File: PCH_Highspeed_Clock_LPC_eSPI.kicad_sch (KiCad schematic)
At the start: 1 part

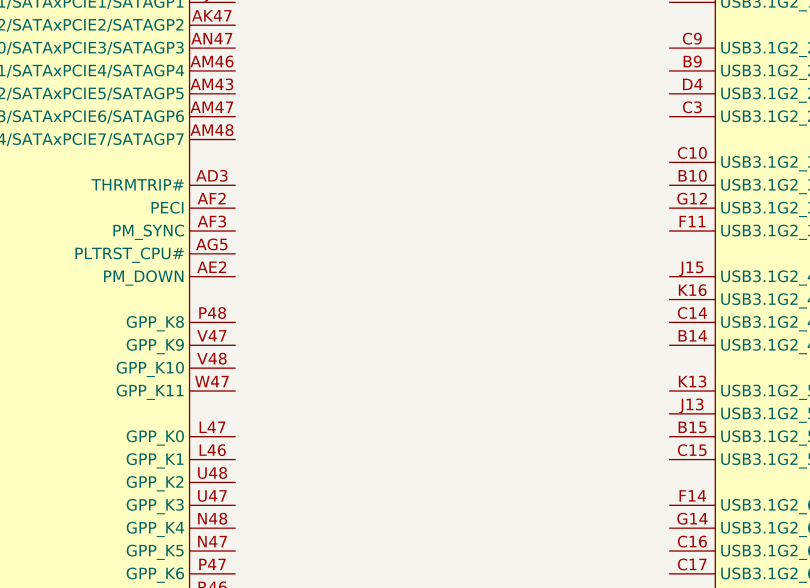
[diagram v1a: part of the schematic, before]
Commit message: implemented some misc cpu signals
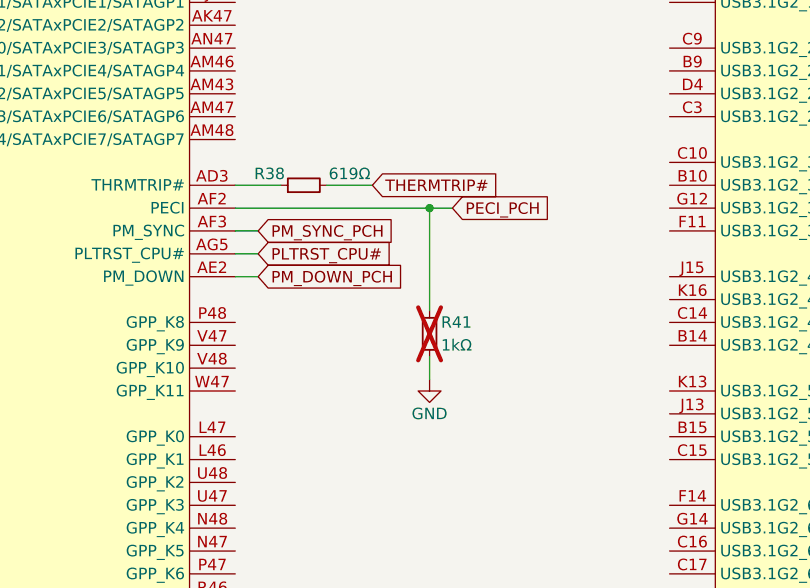
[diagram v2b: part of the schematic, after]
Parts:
- added R38: 619Ω, Resistor_SMD:R_0402_1005Metric, symbol Device:R_Small
- added R41: 1kΩ, Resistor_SMD:R_0402_1005Metric, symbol Device:R_Small
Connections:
- net at UPCH1.AD3 (THRMTRIP#): now also R38.1
- net PM_DOWN_PCH: now reaches UPCH1.AE2 (PM_DOWN)
- net PECI_PCH: now reaches UPCH1.AF2 (PECI)
- net PECI_PCH: now also R41.2
- net PM_SYNC_PCH: now reaches UPCH1.AF3 (PM_SYNC)
- net PLTRST_CPU#: now reaches UPCH1.AG5 (PLTRST_CPU#)
- new net GND: R41.1
- new net THERMTRIP#: R38.2

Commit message: idek what i changed anymore but there's a bunch of new stuff lol
iirc i did some more misc cpu pins and a bunch of pch pcie stuff
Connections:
- net SSD0_Refclk+: now reaches UPCH1.AH10 (CLKOUT_PCIE_P1)
- net SSD0_Refclk-: now reaches UPCH1.AH9 (CLKOUT_PCIE_N1)
- net SSD0_CLKREQ#: now reaches UPCH1.BE31 (GPP_B6/SRCCLKREQ1#)
- net SSD0_PCIe_Tx2+: now reaches UPCH1.B35 (PCIE10_TXP)
- net SSD0_PCIe_Tx1-: now reaches UPCH1.B36 (PCIE11_TXN/SATA0A_TXN)
- net SSD0_PCIe_Tx3-: now reaches UPCH1.C34 (PCIE9_TXN)
- net SSD0_PCIe_Tx2-: now reaches UPCH1.C35 (PCIE10_TXN)
- net SSD0_PCIe_Tx1+: now reaches UPCH1.C36 (PCIE11_TXP/SATA0A_TXP)
- net SSD0_PCIe_Tx3+: now reaches UPCH1.D34 (PCIE9_TXP)
- net SSD0_PCIe/SATA_Tx0-: now reaches UPCH1.D38 (PCIE12_TXN/SATA1A_TXN)
- net SSD0_PCIe/SATA_Tx0+: now reaches UPCH1.E37 (PCIE12_TXP/SATA1A_TXP)
- net SSD0_PCIe_Rx3+: now reaches UPCH1.F36 (PCIE9_RXP)
- net SSD0_PCIe_Rx1+: now reaches UPCH1.F39 (PCIE11_RXP/SATA0A_RXP)
- net SSD0_PCIe_Rx3-: now reaches UPCH1.G36 (PCIE9_RXN)
- net SSD0_PCIe_Rx1-: now reaches UPCH1.G38 (PCIE11_RXN/SATA0A_RXN)
- net SSD0_PCIe/SATA_Rx0-: now reaches UPCH1.H42 (PCIE12_RXN/SATA1A_RXN)
- net SSD0_PCIe_Rx2+: now reaches UPCH1.J37 (PCIE10_RXP)
- net SSD0_PCIe/SATA_Rx0+: now reaches UPCH1.J41 (PCIE12_RXP/SATA1A_RXP)
- net SSD0_PCIe_Rx2-: now reaches UPCH1.K37 (PCIE10_RXN)
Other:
- note added: "PCIe controller 1 (L1-4): ? PCIe controller 2 (L5-8): ? PCIe controller 3 (L9-12): NVMe 0 with lane reversal for SATA on first lane x2 no SATA on H310, x4 with SATA on all other chipsets PCIe controller 4 (L13-16): ? PCIe controller 5 (L17-20): ? PCIe controller 6 (L21-24): ?"
- note added: "subtract 5 for PCIe lane number (first 6 lanes are the USB3.2G2 ports + index starts at 0 vs 1)"
- moved on the sheet: R38, R41, UPCH1G
